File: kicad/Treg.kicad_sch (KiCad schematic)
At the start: 44 parts, among them J1 Conn_01x02, J2 Conn_01x02, J3 Conn_01x02, J4 Conn_01x02, J5 Conn_01x02, J7 Conn_01x07, J8 Conn_01x07, J9 Conn_01x02, U1 PMW3360, U2 TPS73601DBV, U3 XIAO-ESP32-C6-SMD

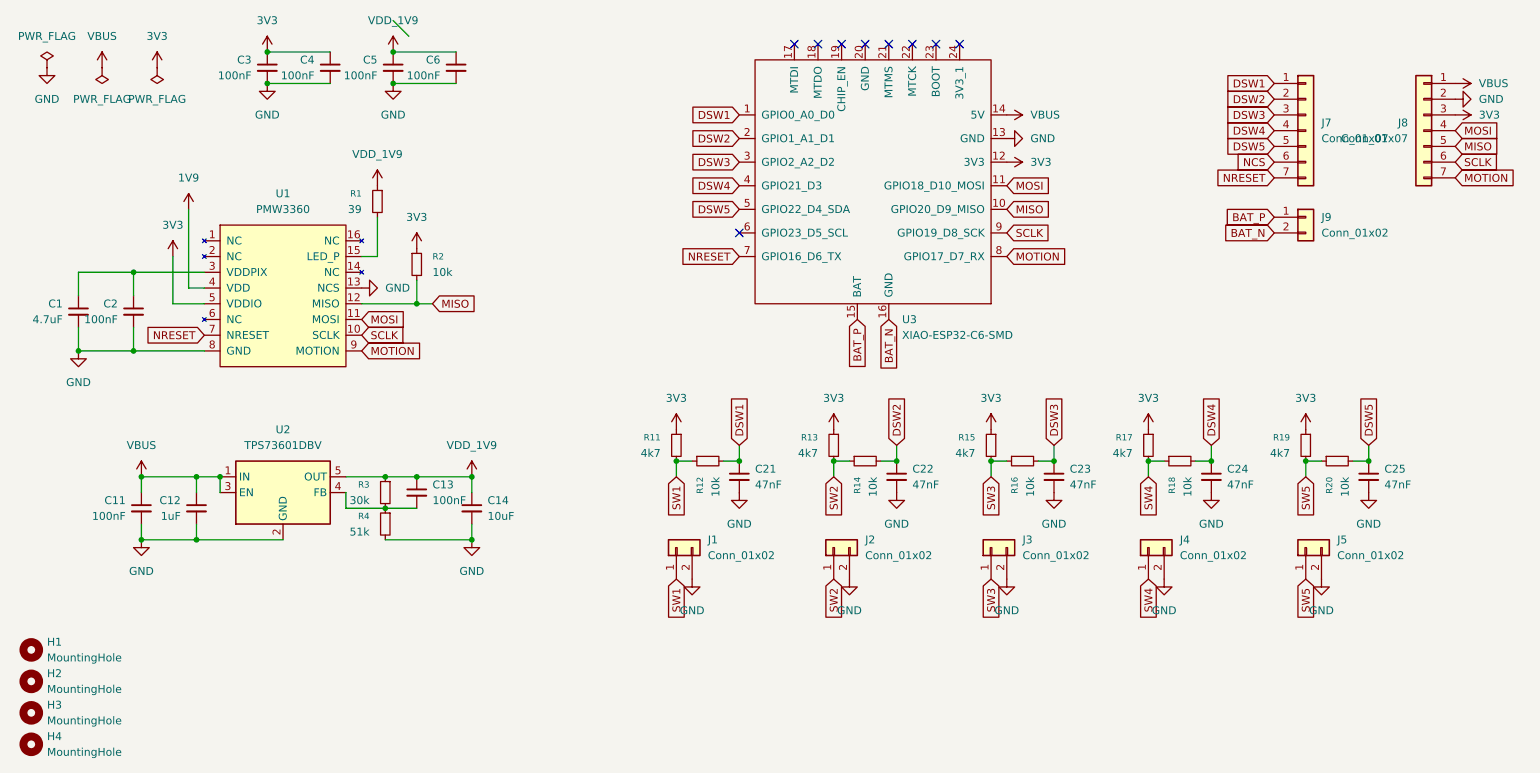
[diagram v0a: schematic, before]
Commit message: wiring gnd
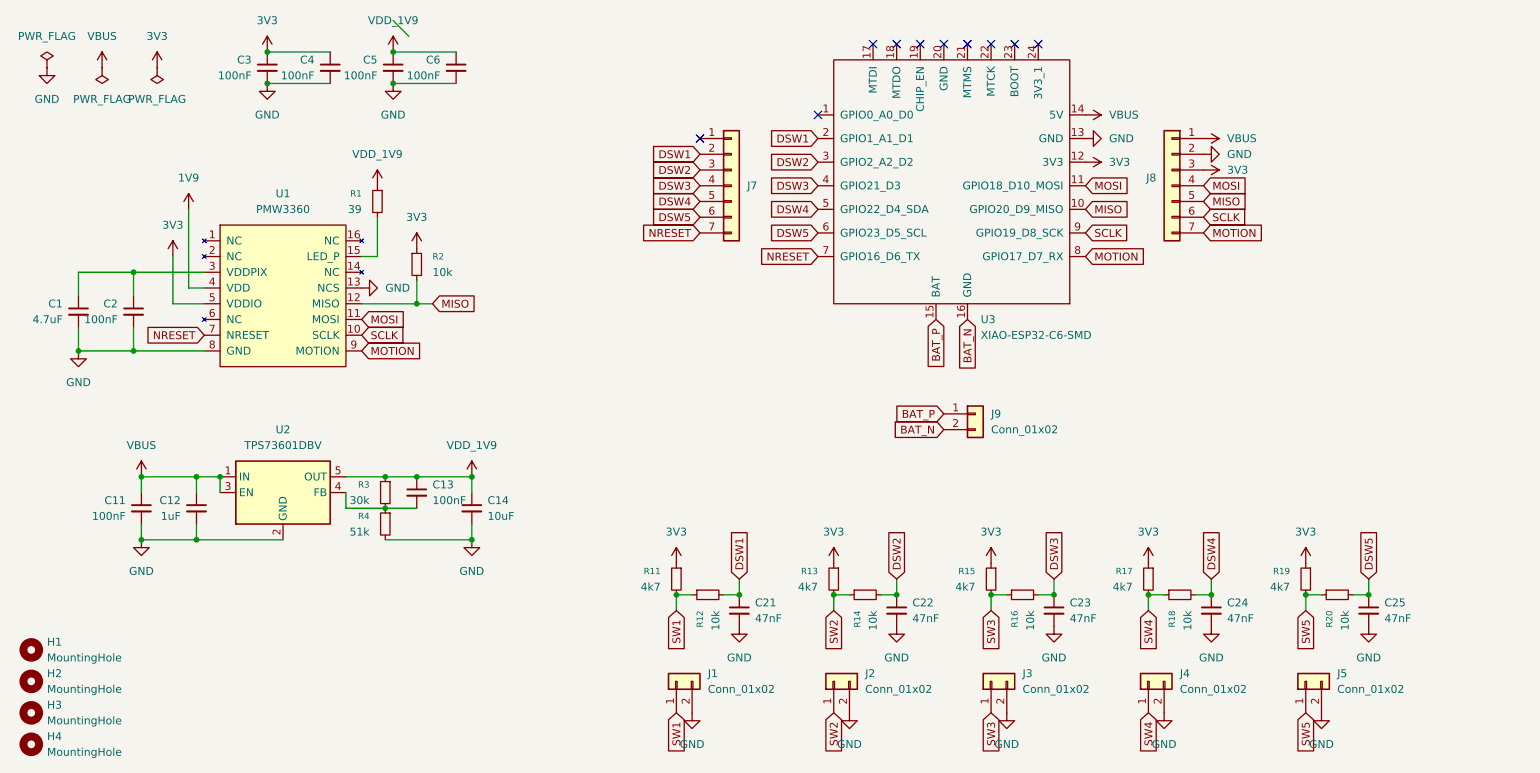
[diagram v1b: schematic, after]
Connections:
- net NCS is gone; now on net DSW5: J7.6 (Pin_6)
- net DSW1: now also J7.2 (Pin_2), U3.2 (GPIO1_A1_D1); no longer J7.1 (Pin_1), U3.1 (GPIO0_A0_D0)
- net DSW2: now also J7.3 (Pin_3), U3.3 (GPIO2_A2_D2); no longer J7.2 (Pin_2), U3.2 (GPIO1_A1_D1)
- net DSW3: now also J7.4 (Pin_4), U3.4 (GPIO21_D3); no longer J7.3 (Pin_3), U3.3 (GPIO2_A2_D2)
- net DSW4: now also J7.5 (Pin_5), U3.5 (GPIO22_D4_SDA); no longer J7.4 (Pin_4), U3.4 (GPIO21_D3)
- net DSW5: now also U3.6 (GPIO23_D5_SCL); no longer J7.5 (Pin_5), U3.5 (GPIO22_D4_SDA)
- no-connect marks 9 -> 10
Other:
- moved on the sheet: C21, C22, C23, C24, C25, J1, J2, J3, J4, J5, J7, J8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
